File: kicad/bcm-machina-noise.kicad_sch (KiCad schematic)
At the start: 61 parts, among them J1 USB_A, J2 AVR-ISP-6, J3 AudioJack2_SwitchT, J5 AudioJack2_SwitchT, Q1 2N5457, Q2 2N5457, SW1 SW_Push, SW2 SW_Push, U1 4069, U2 MCP602, U3 ATtiny84V-10P

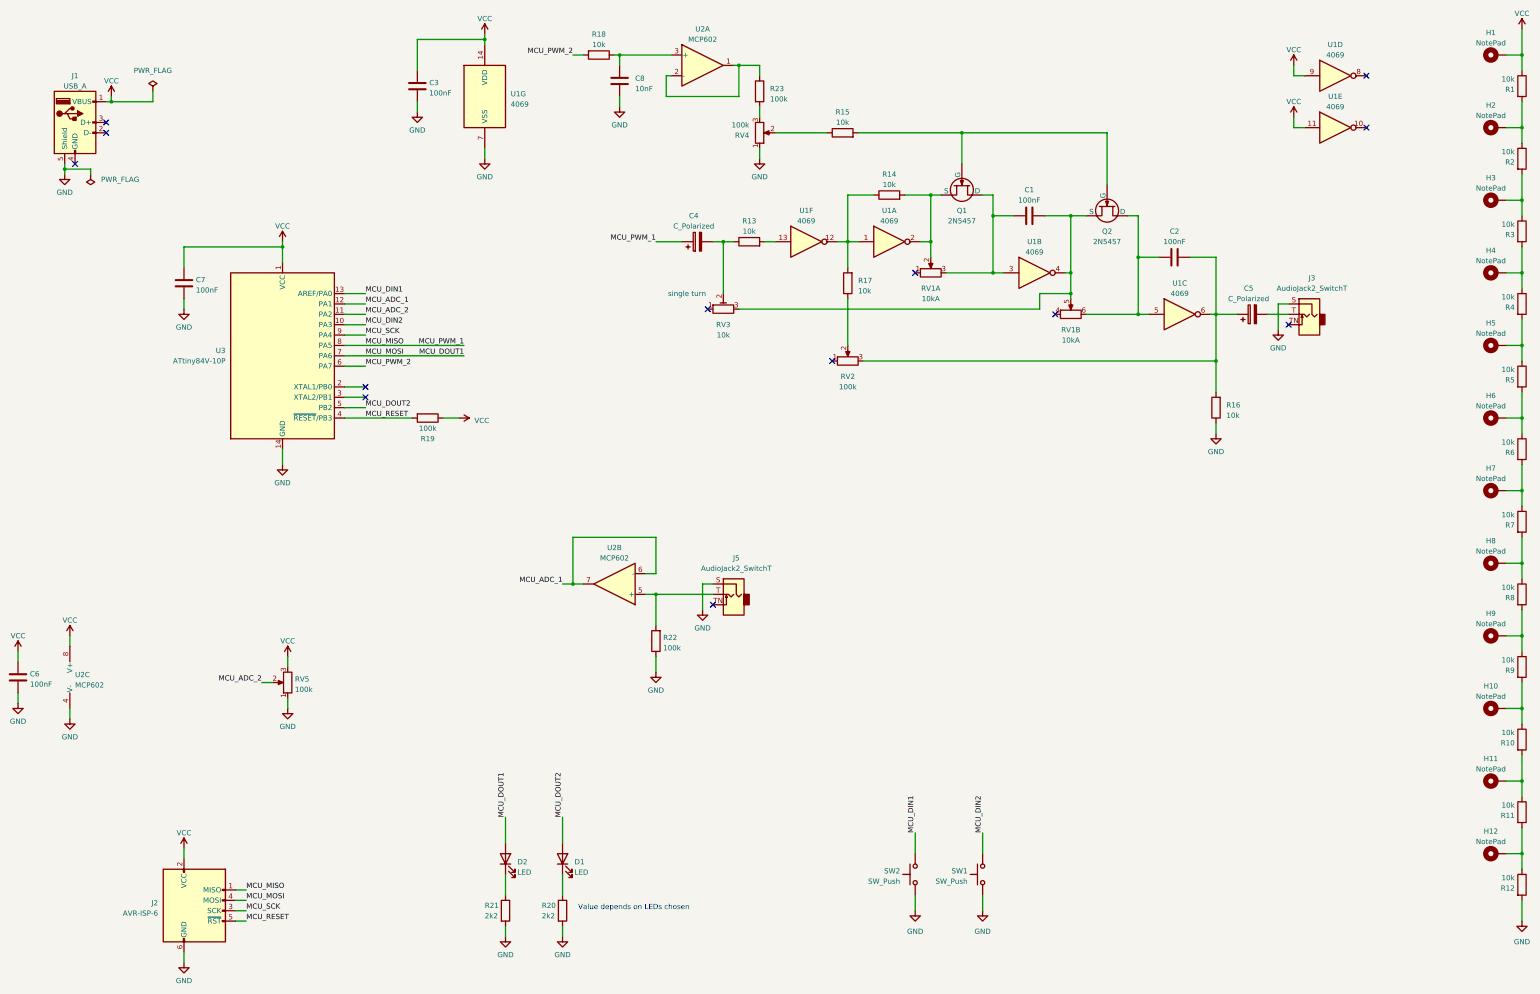
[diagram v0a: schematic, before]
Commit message: Updating schematic with fixes and changes
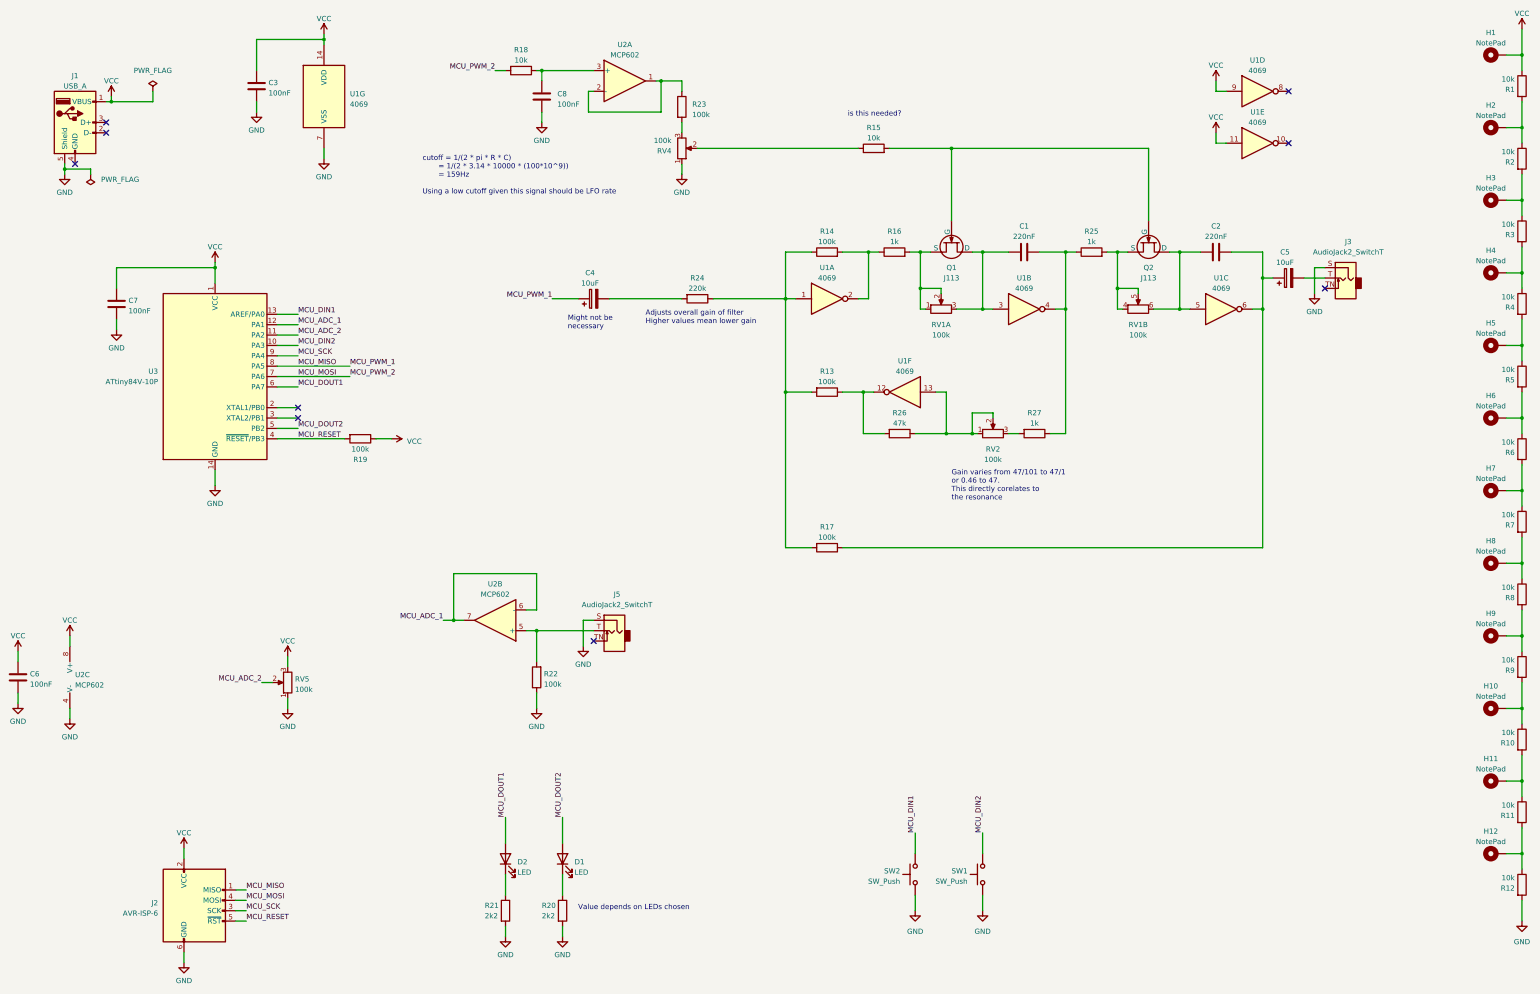
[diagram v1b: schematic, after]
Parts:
- removed RV3: 10k, Trimpot:Potentiometer_THT_Bourns_3306P_Vertical, symbol Device:R_Potentiometer_Trim
- added R24: 220k, Resistor_THT:R_Axial_DIN0207_L6.3mm_D2.5mm_P10.16mm_Horizontal, symbol Device:R
- added R25, R27: 1k, Resistor_THT:R_Axial_DIN0207_L6.3mm_D2.5mm_P10.16mm_Horizontal, symbol Device:R
- added R26: 47k, Resistor_THT:R_Axial_DIN0207_L6.3mm_D2.5mm_P10.16mm_Horizontal, symbol Device:R
- C1, C2: value 100nF -> 220nF
- C4, C5: value C_Polarized -> 10uF
- C8: value 10nF -> 100nF
- Q1, Q2: value 2N5457 -> J113
- R13, R14, R17: value 10k -> 100k
- R16: value 10k -> 1k
- RV1: value 10kA -> 100k
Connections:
- net GND: no longer R16.1
- net MCU_DOUT1: now also U3.6 (PA7); no longer J2.4 (MOSI), U3.7 (PA6)
- net at C1.2, U1.4: now also R25.1, R27.1; no longer Q2.3 (S), RV1.5
- net at R14.1, R17.2, U1.1: now also R13.2, R24.1; no longer U1.12
- net at R14.2, U1.2: now also R16.1; no longer Q1.3 (S), RV1.2
- net at C2.2, C5.1, U1.6: now also R17.1; no longer R16.2, RV2.3
- net at C4.2: now also R24.2; no longer R13.1
- net at U1.13: now also RV2.1, RV2.2, R26.1; no longer R13.2
- net at RV1.4: now also Q2.3 (S), RV1.5, R25.2
- net at RV1.1: now also Q1.3 (S), R16.2, RV1.2
- net MCU_PWM_2 renamed MCU_MOSI
- net MCU_MOSI: now also J2.4 (MOSI), U3.7 (PA6); no longer U3.6 (PA7)
- new net: R27.2, RV2.3
- new net: R13.1, R26.2, U1.12
- no-connect marks 13 -> 9
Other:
- note added: "Adjusts overall gain of filter Higher values mean lower gain"
- note added: "Gain varies from 47/101 to 47/1 or 0.46 to 47. This directly corelates to the resonance"
- note added: "Might not be necessary"
- note added: "cutoff = 1/(2 * pi * R * C) = 1/(2 * 3.14 * 10000 * (100*10^9)) = 159Hz Using a low cutoff given this signal should be LFO rate"
- note added: "is this needed?"
- moved on the sheet: C1, C2, C3, C4, C5, C7, C8, J3, J5, Q1, Q2, R13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
